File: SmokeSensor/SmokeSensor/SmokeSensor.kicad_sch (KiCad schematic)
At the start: 0 parts

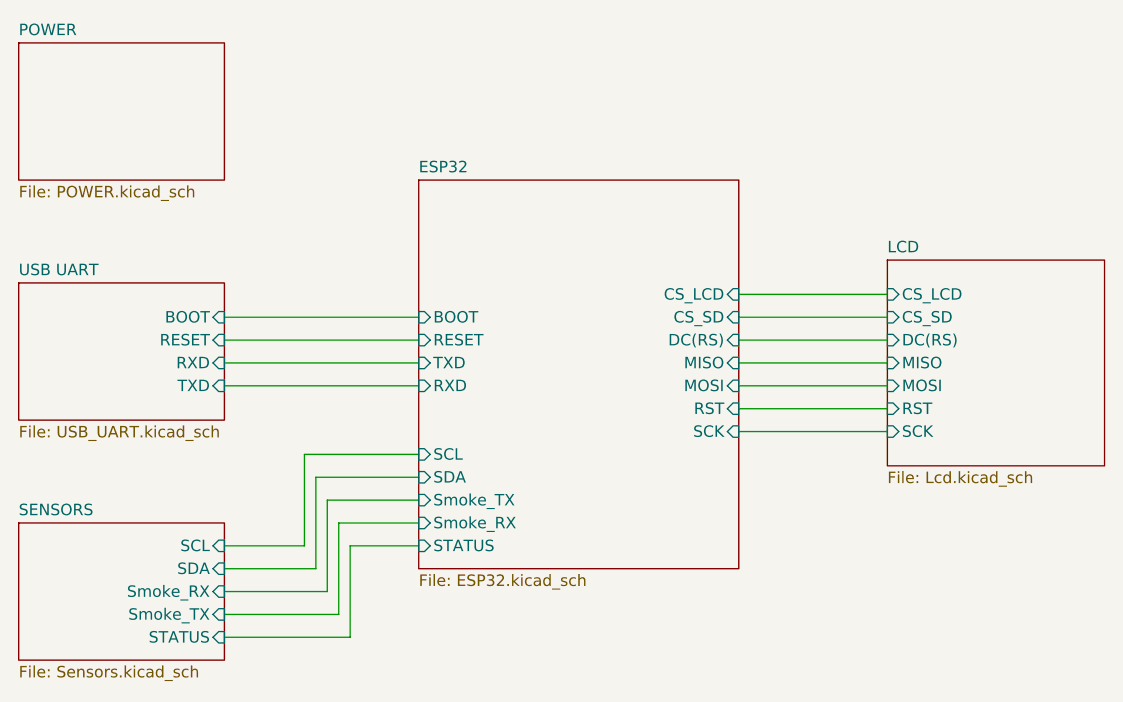
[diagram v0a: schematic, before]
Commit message: layout 2-layers done!
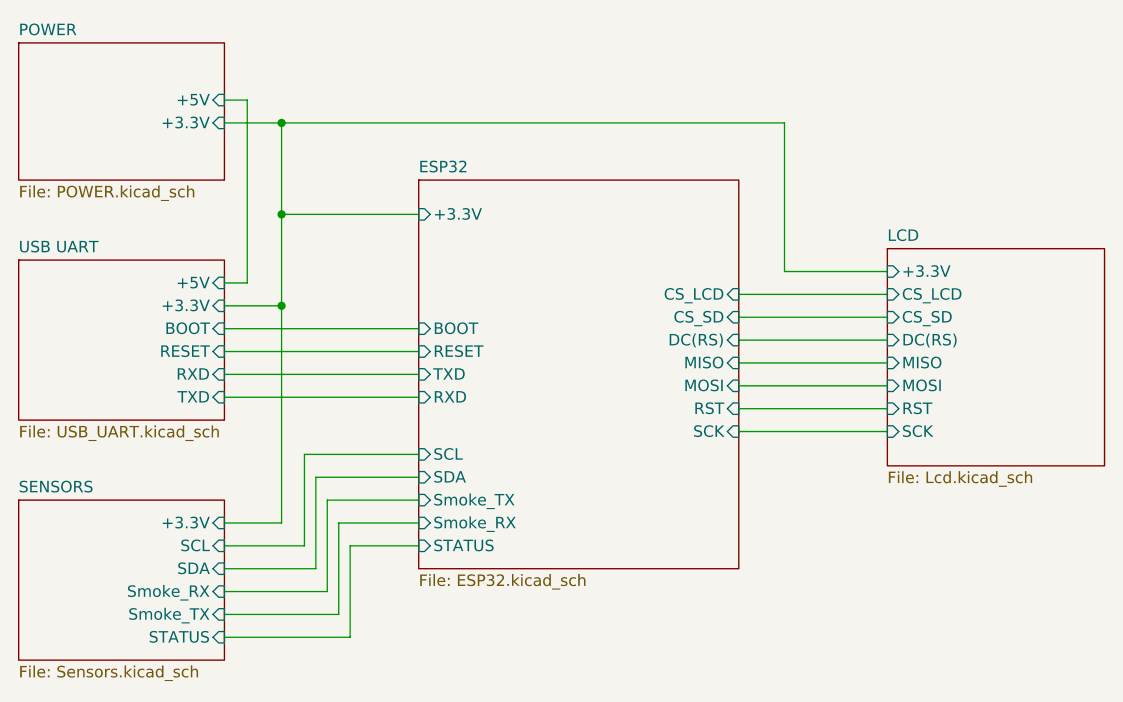
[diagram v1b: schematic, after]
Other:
- sheet ESP32 ports: added +3.3V; removed none
- sheet LCD ports: added +3.3V; removed none
- sheet POWER ports: added +3.3V, +5V; removed none
- sheet SENSORS ports: added +3.3V; removed none
- sheet USB UART ports: added +3.3V, +5V; removed none
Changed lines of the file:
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@@
 		(date "2026-04-08")
 	)
-	(wire
-		(pts
-			(xy 110.49 85.09) (xy 132.08 85.09)
+	(junction
+		(at 116.84 63.5)
+		(diameter 0)
+		(color 0 0 0 0)
+	)
+	(junction
+		(at 116.84 83.82)
+		(diameter 0)
+		(color 0 0 0 0)
+	)
+	(junction
+		(at 116.84 73.66)
+		(diameter 0)
+		(color 0 0 0 0)
+	)
+	(wire
+		(pts
+			(xy 110.49 86.36) (xy 132.08 86.36)
 		)
 		(stroke
@@
 	(wire
 		(pts
-			(xy 110.49 87.63) (xy 132.08 87.63)
+			(xy 110.49 88.9) (xy 132.08 88.9)
+		)
+		(stroke
+			(width 0)
+			(type default)
+		)
+	)
+	(wire
+		(pts
+			(xy 184.15 80.01) (xy 172.72 80.01)
+		)
+		(stroke
+			(width 0)
+			(type default)
+		)
+	)
+	(wire
+		(pts
+			(xy 113.03 60.96) (xy 113.03 81.28)
+		)
+		(stroke
+			(width 0)
+			(type default)
+		)
+	)
+	(wire
+		(pts
+			(xy 116.84 83.82) (xy 116.84 107.95)
+		)
+		(stroke
+			(width 0)
+			(type default)
+		)
+	)
+	(wire
+		(pts
+			(xy 113.03 81.28) (xy 110.49 81.28)
 		)
 		(stroke
@@
 	(wire
 		(pts
+			(xy 172.72 80.01) (xy 172.72 63.5)
+		)
+		(stroke
+			(width 0)
+			(type default)
+		)
+	)
+	(wire
+		(pts
 			(xy 167.64 82.55) (xy 184.15 82.55)
 		)
@@
 	(wire
 		(pts
+			(xy 116.84 63.5) (xy 116.84 73.66)
+		)
+		(stroke
+			(width 0)
+			(type default)
+		)
+	)
+	(wire
+		(pts
 			(xy 120.65 113.03) (xy 110.49 113.03)
 		)
@@
 	(wire
 		(pts
-			(xy 110.49 90.17) (xy 132.08 90.17)
+			(xy 110.49 91.44) (xy 132.08 91.44)
+		)
+		(stroke
+			(width 0)
+			(type default)
+		)
+	)
+	(wire
+		(pts
+			(xy 116.84 73.66) (xy 132.08 73.66)
 		)
 		(stroke
@@
 	(wire
 		(pts
+			(xy 172.72 63.5) (xy 116.84 63.5)
+		)
+		(stroke
+			(width 0)
+			(type default)
+		)
+	)
+	(wire
+		(pts
 			(xy 132.08 107.95) (xy 123.19 107.95)
 		)
@@
 	(wire
 		(pts
-			(xy 110.49 92.71) (xy 132.08 92.71)
+			(xy 110.49 93.98) (xy 132.08 93.98)
+		)
+		(stroke
+			(width 0)
+			(type default)
+		)
+	)
+	(wire
+		(pts
+			(xy 110.49 63.5) (xy 116.84 63.5)
+		)
+		(stroke
+			(width 0)
+			(type default)
+		)
+	)
+	(wire
+		(pts
+			(xy 116.84 107.95) (xy 110.49 107.95)
+		)
+		(stroke
+			(width 0)
+			(type default)
+		)
+	)
+	(wire
+		(pts
+			(xy 110.49 83.82) (xy 116.84 83.82)
 		)
 		(stroke
@@
 	(wire
 		(pts
+			(xy 116.84 73.66) (xy 116.84 83.82)
+		)
+		(stroke
+			(width 0)
+			(type default)
+		)
+	)
+	(wire
+		(pts
 			(xy 167.64 87.63) (xy 184.15 87.63)
 		)
@@
 		(pts
 			(xy 167.64 95.25) (xy 184.15 95.25)
+		)
+		(stroke
+			(width 0)
+			(type default)
+		)
+	)
+	(wire
+		(pts
+			(xy 110.49 60.96) (xy 113.03 60.96)
 		)
 		(stroke
@@
 			)
 		)
+		(pin "+3.3V" input
+			(at 110.49 63.5 0)
+			(effects
+				(font
+					(size 1.27 1.27)
+				)
+				(justify right)
+			)
+		)
+		(pin "+5V" input
+			(at 110.49 60.96 0)
+			(effects
+				(font
+					(size 1.27 1.27)
+				)
+				(justify right)
+			)
+		)
 		(instances
 			(project "SmokeSensor"
@@
 		)
 		(pin "RXD" input
-			(at 132.08 92.71 180)
+			(at 132.08 93.98 180)
 			(effects
 				(font
@@
 		)
 		(pin "TXD" input
-			(at 132.08 90.17 180)
+			(at 132.08 91.44 180)
 			(effects
 				(font
@@
 		)
 		(pin "BOOT" input
-			(at 132.08 85.09 180)
+			(at 132.08 86.36 180)
 			(effects
 				(font
@@
 		)
 		(pin "RESET" input
-			(at 132.08 87.63 180)
+			(at 132.08 88.9 180)
 			(effects
 				(font
@@
 				)
 				(justify right)
+			)
+		)
+		(pin "+3.3V" input
+			(at 132.08 73.66 180)
+			(effects
+				(font
+					(size 1.27 1.27)
+				)
+				(justify left)
 			)
 		)
@@
 	)
 	(sheet
-		(at 87.63 107.95)
-		(size 22.86 15.24)
+		(at 87.63 105.41)
+		(size 22.86 17.78)
 		(exclude_from_sim no)
 		(in_bom yes)
@@
 		)
 		(property "Sheetname" "SENSORS"
-			(at 87.63 107.2384 0)
+			(at 87.63 104.6984 0)
 			(effects
 				(font
@@
 		(pin "STATUS" input
 			(at 110.49 120.65 0)
+			(effects
+				(font
+					(size 1.27 1.27)
+				)
+				(justify right)
+			)
+		)
+		(pin "+3.3V" input
+			(at 110.49 107.95 0)
 			(effects
 				(font
@@
 	)
 	(sheet
-		(at 87.63 81.28)
-		(size 22.86 15.24)
+		(at 87.63 78.74)
+		(size 22.86 17.78)
 		(exclude_from_sim no)
 		(in_bom yes)
@@
 		)
 		(property "Sheetname" "USB UART"
-			(at 87.63 80.5684 0)
+			(at 87.63 78.0284 0)
 			(effects
 				(font
@@
 		)
 		(pin "BOOT" input
-			(at 110.49 85.09 0)
+			(at 110.49 86.36 0)
 			(effects
 				(font
@@
 		)
 		(pin "RESET" input
-			(at 110.49 87.63 0)
+			(at 110.49 88.9 0)
 			(effects
 				(font
@@
 		)
 		(pin "RXD" input
-			(at 110.49 90.17 0)
+			(at 110.49 91.44 0)
 			(effects
 				(font
@@
 		)
 		(pin "TXD" input
-			(at 110.49 92.71 0)
+			(at 110.49 93.98 0)
+			(effects
+				(font
+					(size 1.27 1.27)
+				)
+				(justify right)
+			)
+		)
+		(pin "+3.3V" input
+			(at 110.49 83.82 0)
+			(effects
+				(font
+					(size 1.27 1.27)
+				)
+				(justify right)
+			)
+		)
+		(pin "+5V" input
+			(at 110.49 81.28 0)
 			(effects
 				(font
@@
 	)
 	(sheet
-		(at 184.15 78.74)
-		(size 24.13 22.86)
+		(at 184.15 77.47)
+		(size 24.13 24.13)
 		(exclude_from_sim no)
 		(in_bom yes)
@@
 		)
 		(property "Sheetname" "LCD"
-			(at 184.15 78.0284 0)
+			(at 184.15 76.7584 0)
 			(effects
 				(font
@@
 			(effects
 				(font
+					(size 1.27 1.27)
+				)
+				(justify left)
+			)
+		)
+		(pin "+3.3V" input
+			(at 184.15 80.01 180)
+			(effects
+				(font
